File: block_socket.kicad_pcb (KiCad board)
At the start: 2 copper layers, 40 x 40 mm, 16 parts, among them J401 Conn_01x03_Pin, J402 Conn_01x03_Pin, J403 Conn_01x03_Pin, J404 Conn_01x03_Pin, J405 Pogopin_pad, J406 Pogopin_pad, J407 Pogopin_pad, J408 Pogopin_pad, J409 Pogopin_pad, J410 Pogopin_pad, J411 Pogopin_pad, J412 Pogopin_pad

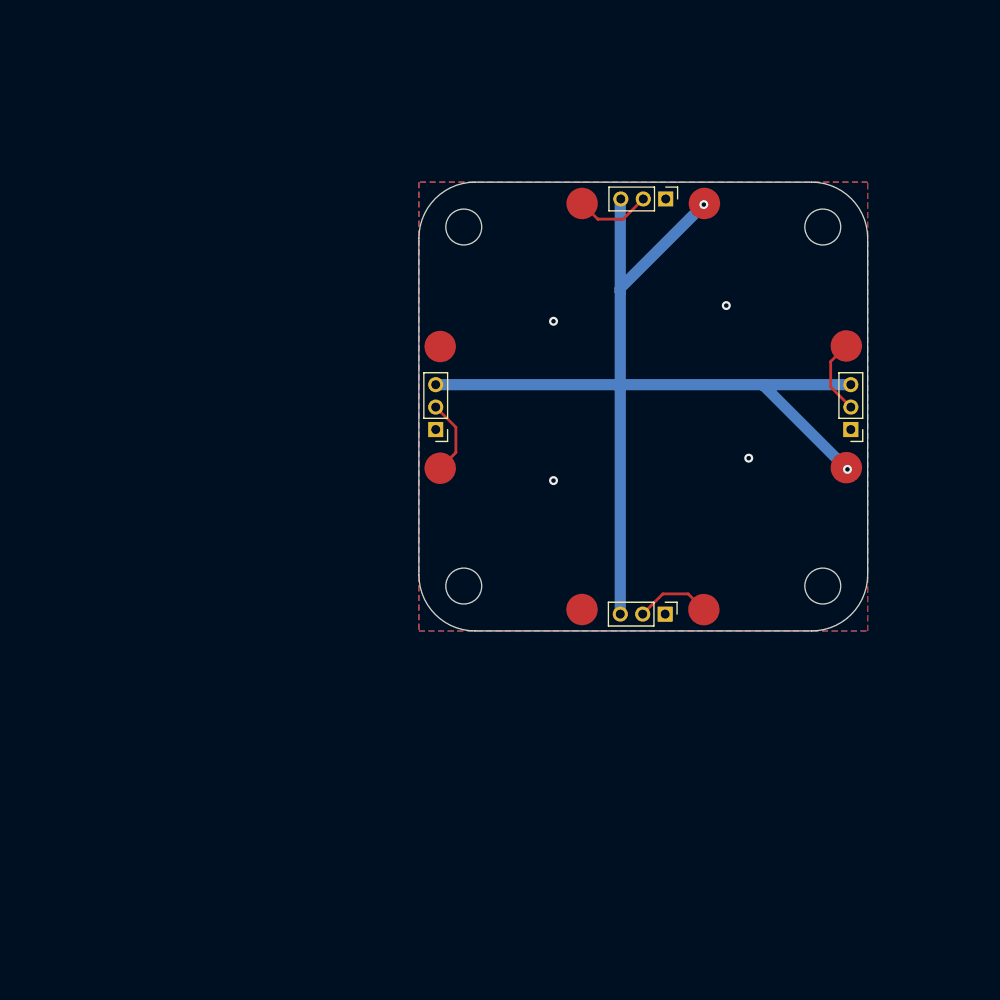
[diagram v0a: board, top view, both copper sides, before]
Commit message: gerber
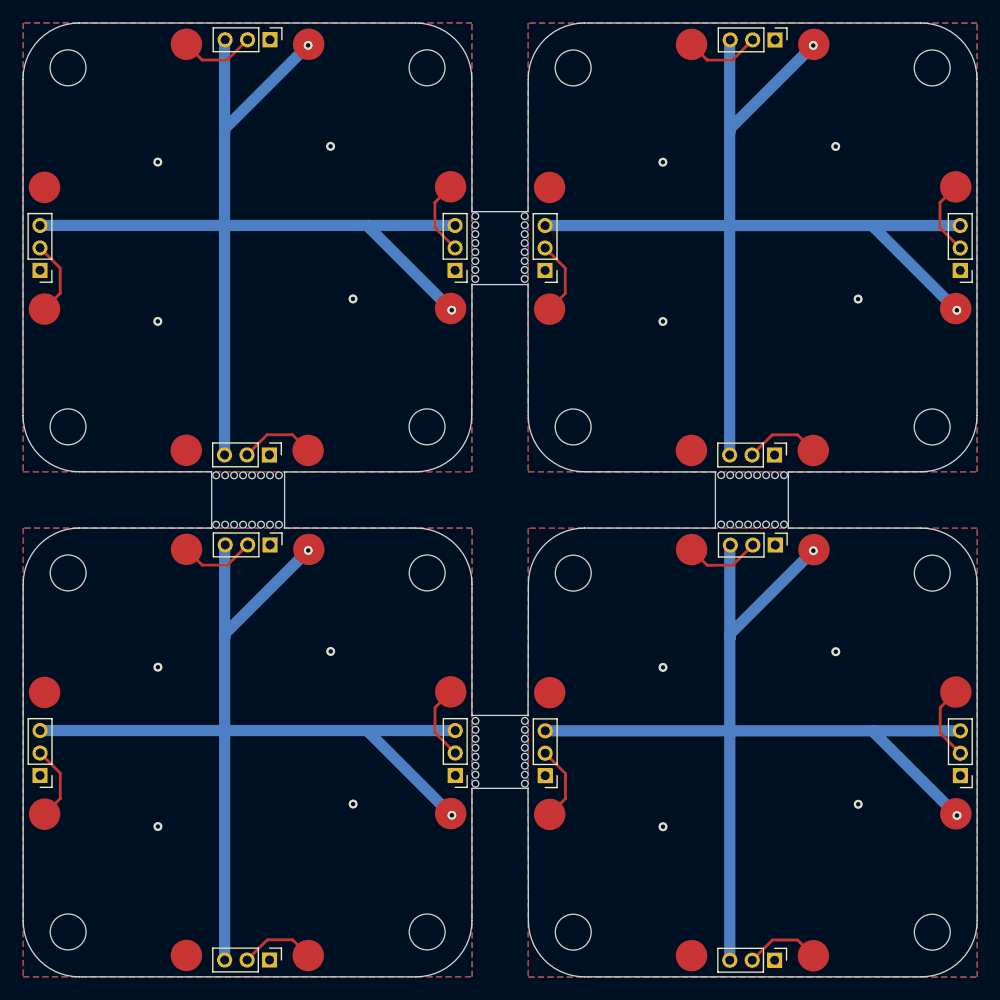
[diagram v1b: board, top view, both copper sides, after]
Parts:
- removed the J401 at (122.0, 51.5)
- removed the J402 at (138.5, 72.0)
- removed the J403 at (122.0, 88.5)
- removed the J404 at (101.5, 72.0)
- removed the J405 at (114.5, 51.9)
- removed the J406 at (138.1, 64.6)
- removed the J407 at (125.4, 88.1)
- removed the J408 at (101.9, 75.5)
- removed the J409 at (125.5, 51.9)
- removed the J410 at (138.1, 75.5)
- removed the J411 at (114.5, 88.1)
- removed the J412 at (101.9, 64.7)
- removed the REF** at (136.0, 54.0)
- removed the REF** at (104.0, 54.0)
- removed the REF** at (136.0, 86.0)
- removed the REF** at (104.0, 86.0)
- added J401: Conn_01x03_Pin, Connector_PinHeader_2.00mm:PinHeader_1x03_P2.00mm_Vertical, F.Cu at (131.8, 37.3)
- added J401: Conn_01x03_Pin, Connector_PinHeader_2.00mm:PinHeader_1x03_P2.00mm_Vertical, F.Cu at (86.7, 82.3)
- added J401: Conn_01x03_Pin, Connector_PinHeader_2.00mm:PinHeader_1x03_P2.00mm_Vertical, F.Cu at (86.7, 37.3)
- added J401: Conn_01x03_Pin, Connector_PinHeader_2.00mm:PinHeader_1x03_P2.00mm_Vertical, F.Cu at (131.8, 82.3)
- added J402: Conn_01x03_Pin, Connector_PinHeader_2.00mm:PinHeader_1x03_P2.00mm_Vertical, F.Cu at (148.2, 57.9)
- added J402: Conn_01x03_Pin, Connector_PinHeader_2.00mm:PinHeader_1x03_P2.00mm_Vertical, F.Cu at (103.2, 102.9)
- added J402: Conn_01x03_Pin, Connector_PinHeader_2.00mm:PinHeader_1x03_P2.00mm_Vertical, F.Cu at (103.2, 57.9)
- added J402: Conn_01x03_Pin, Connector_PinHeader_2.00mm:PinHeader_1x03_P2.00mm_Vertical, F.Cu at (148.3, 102.9)
- added J403: Conn_01x03_Pin, Connector_PinHeader_2.00mm:PinHeader_1x03_P2.00mm_Vertical, F.Cu at (86.7, 74.3)
- added J403: Conn_01x03_Pin, Connector_PinHeader_2.00mm:PinHeader_1x03_P2.00mm_Vertical, F.Cu at (131.7, 119.3)
- added J403: Conn_01x03_Pin, Connector_PinHeader_2.00mm:PinHeader_1x03_P2.00mm_Vertical, F.Cu at (86.7, 119.3)
- added J403: Conn_01x03_Pin, Connector_PinHeader_2.00mm:PinHeader_1x03_P2.00mm_Vertical, F.Cu at (131.7, 74.3)
- added J404: Conn_01x03_Pin, Connector_PinHeader_2.00mm:PinHeader_1x03_P2.00mm_Vertical, F.Cu at (111.3, 102.9)
- added J404: Conn_01x03_Pin, Connector_PinHeader_2.00mm:PinHeader_1x03_P2.00mm_Vertical, F.Cu at (111.2, 57.9)
- added J404: Conn_01x03_Pin, Connector_PinHeader_2.00mm:PinHeader_1x03_P2.00mm_Vertical, F.Cu at (66.2, 102.9)
- added J404: Conn_01x03_Pin, Connector_PinHeader_2.00mm:PinHeader_1x03_P2.00mm_Vertical, F.Cu at (66.2, 57.9)
- added J405: Pogopin_pad, LIB:Pogopin_pad, F.Cu at (79.3, 82.7)
- added J405: Pogopin_pad, LIB:Pogopin_pad, F.Cu at (124.3, 82.8)
- added J405: Pogopin_pad, LIB:Pogopin_pad, F.Cu at (124.3, 37.7)
- added J405: Pogopin_pad, LIB:Pogopin_pad, F.Cu at (79.3, 37.7)
- added J406: Pogopin_pad, LIB:Pogopin_pad, F.Cu at (147.9, 95.5)
- added J406: Pogopin_pad, LIB:Pogopin_pad, F.Cu at (102.8, 50.4)
- added J406: Pogopin_pad, LIB:Pogopin_pad, F.Cu at (147.8, 50.4)
- added J406: Pogopin_pad, LIB:Pogopin_pad, F.Cu at (102.8, 95.4)
- added J407: Pogopin_pad, LIB:Pogopin_pad, F.Cu at (90.1, 118.9)
- added J407: Pogopin_pad, LIB:Pogopin_pad, F.Cu at (90.1, 73.9)
- added J407: Pogopin_pad, LIB:Pogopin_pad, F.Cu at (135.2, 119.0)
- added J407: Pogopin_pad, LIB:Pogopin_pad, F.Cu at (135.2, 73.9)
- added J408: Pogopin_pad, LIB:Pogopin_pad, F.Cu at (66.6, 61.3)
- added J408: Pogopin_pad, LIB:Pogopin_pad, F.Cu at (111.7, 106.3)
- added J408: Pogopin_pad, LIB:Pogopin_pad, F.Cu at (66.6, 106.3)
- added J408: Pogopin_pad, LIB:Pogopin_pad, F.Cu at (111.7, 61.3)
- added J409: Pogopin_pad, LIB:Pogopin_pad, F.Cu at (90.2, 37.7)
- added J409: Pogopin_pad, LIB:Pogopin_pad, F.Cu at (135.2, 37.7)
- added J409: Pogopin_pad, LIB:Pogopin_pad, F.Cu at (135.2, 82.8)
- added J409: Pogopin_pad, LIB:Pogopin_pad, F.Cu at (90.2, 82.7)
- added J410: Pogopin_pad, LIB:Pogopin_pad, F.Cu at (102.8, 61.3)
- added J410: Pogopin_pad, LIB:Pogopin_pad, F.Cu at (147.8, 61.3)
- added J410: Pogopin_pad, LIB:Pogopin_pad, F.Cu at (147.9, 106.3)
- added J410: Pogopin_pad, LIB:Pogopin_pad, F.Cu at (102.8, 106.3)
- added J411: Pogopin_pad, LIB:Pogopin_pad, F.Cu at (124.3, 73.9)
- added J411: Pogopin_pad, LIB:Pogopin_pad, F.Cu at (124.3, 118.9)
- added J411: Pogopin_pad, LIB:Pogopin_pad, F.Cu at (79.3, 73.9)
- added J411: Pogopin_pad, LIB:Pogopin_pad, F.Cu at (79.3, 118.9)
- added J412: Pogopin_pad, LIB:Pogopin_pad, F.Cu at (66.6, 95.5)
- added J412: Pogopin_pad, LIB:Pogopin_pad, F.Cu at (111.7, 50.5)
- added J412: Pogopin_pad, LIB:Pogopin_pad, F.Cu at (111.7, 95.5)
- added J412: Pogopin_pad, LIB:Pogopin_pad, F.Cu at (66.6, 50.5)
- added REF**: MountingHole_3.2mm_M3, MountingHole:MountingHole_3.2mm_M3, F.Cu at (68.7, 84.8)
- added REF**: bridge, LIB:bridge, F.Cu at (81.5, 75.8)
- added REF**: MountingHole_3.2mm_M3, MountingHole:MountingHole_3.2mm_M3, F.Cu at (113.8, 84.8)
- added REF**: MountingHole_3.2mm_M3, MountingHole:MountingHole_3.2mm_M3, F.Cu at (145.8, 84.8)
- added REF**: bridge, LIB:bridge, F.Cu at (104.7, 104.0)
- added REF**: bridge, LIB:bridge, F.Cu at (132.9, 80.8)
- added REF**: MountingHole_3.2mm_M3, MountingHole:MountingHole_3.2mm_M3, F.Cu at (145.8, 116.8)
- added REF**: MountingHole_3.2mm_M3, MountingHole:MountingHole_3.2mm_M3, F.Cu at (100.7, 71.8)
- added REF**: MountingHole_3.2mm_M3, MountingHole:MountingHole_3.2mm_M3, F.Cu at (100.7, 39.8)
- added REF**: MountingHole_3.2mm_M3, MountingHole:MountingHole_3.2mm_M3, F.Cu at (113.8, 39.8)
- added REF**: MountingHole_3.2mm_M3, MountingHole:MountingHole_3.2mm_M3, F.Cu at (100.7, 116.8)
- added REF**: MountingHole_3.2mm_M3, MountingHole:MountingHole_3.2mm_M3, F.Cu at (113.8, 116.8)
- added REF**: MountingHole_3.2mm_M3, MountingHole:MountingHole_3.2mm_M3, F.Cu at (100.7, 84.8)
- added REF**: MountingHole_3.2mm_M3, MountingHole:MountingHole_3.2mm_M3, F.Cu at (68.7, 116.8)
- added REF**: MountingHole_3.2mm_M3, MountingHole:MountingHole_3.2mm_M3, F.Cu at (68.7, 71.8)
- added REF**: bridge, LIB:bridge, F.Cu at (109.7, 52.6)
- added REF**: MountingHole_3.2mm_M3, MountingHole:MountingHole_3.2mm_M3, F.Cu at (145.8, 71.8)
- added REF**: MountingHole_3.2mm_M3, MountingHole:MountingHole_3.2mm_M3, F.Cu at (113.8, 71.8)
- added REF**: MountingHole_3.2mm_M3, MountingHole:MountingHole_3.2mm_M3, F.Cu at (68.7, 39.8)
- added REF**: MountingHole_3.2mm_M3, MountingHole:MountingHole_3.2mm_M3, F.Cu at (145.8, 39.8)
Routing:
- net +5V: track 95.5 -> 382.1 mm, vias 2 -> 8
- net S_S: track 6.78 -> 27.1 mm
- net W_S: track 6.78 -> 27.1 mm
- net E_S: track 6.78 -> 27.1 mm
- net N_S: track 6.78 -> 27.1 mm
- net GND: vias 4 -> 16
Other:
- board size 40 x 40 mm -> 85 x 85 mm
